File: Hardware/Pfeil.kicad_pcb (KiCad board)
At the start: 4 copper layers, 50 x 6 mm, 62 parts, among them IC1 2536030320001, IC2 nPM1300-CAAA-R, J1 Conn_01x01_Socket, J2 Conn_01x01_Socket, J3 TagConnect, U1 NRF52840-CKAA-R, U2 WSEN-PADS_2511020213301, U3 WSEN-PADS_2511020213301, X1 XTAL 32MHz 8pF, X2 XTAL 32.768kHz 9pF

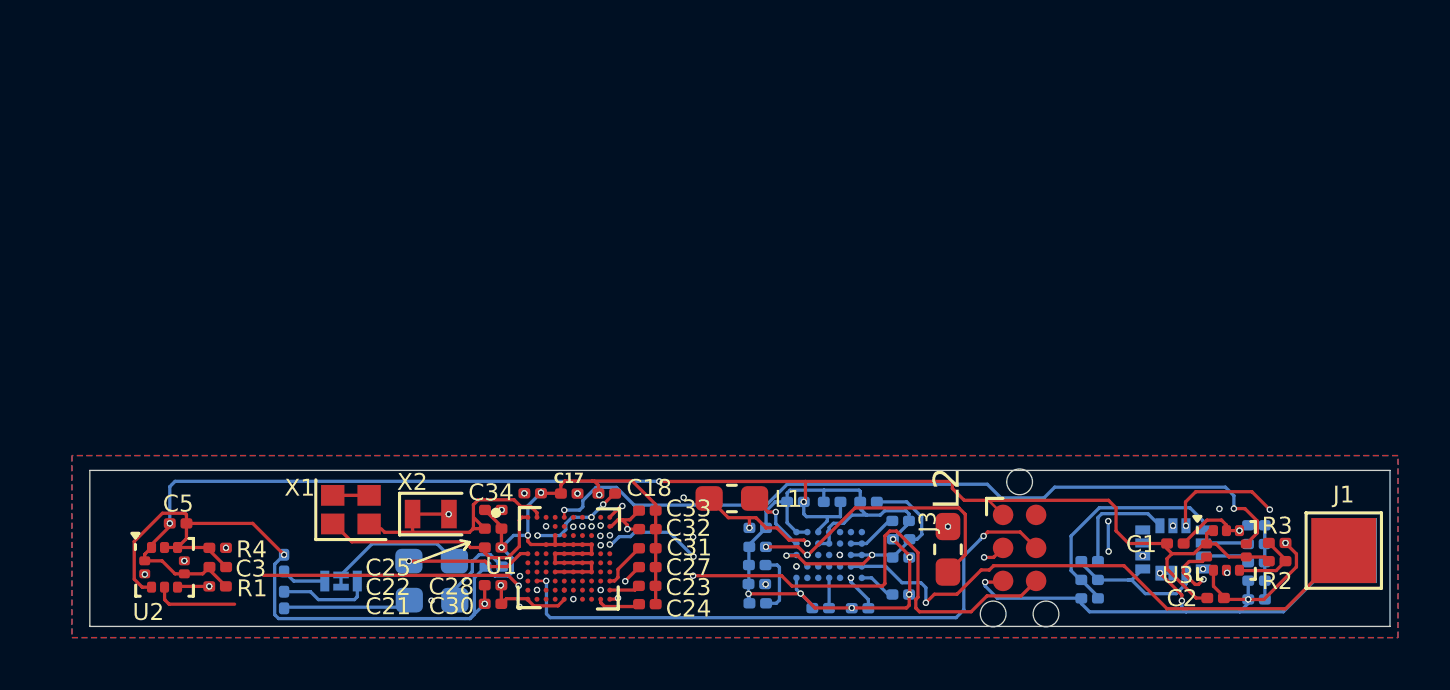
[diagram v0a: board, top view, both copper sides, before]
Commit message: Fix some shit
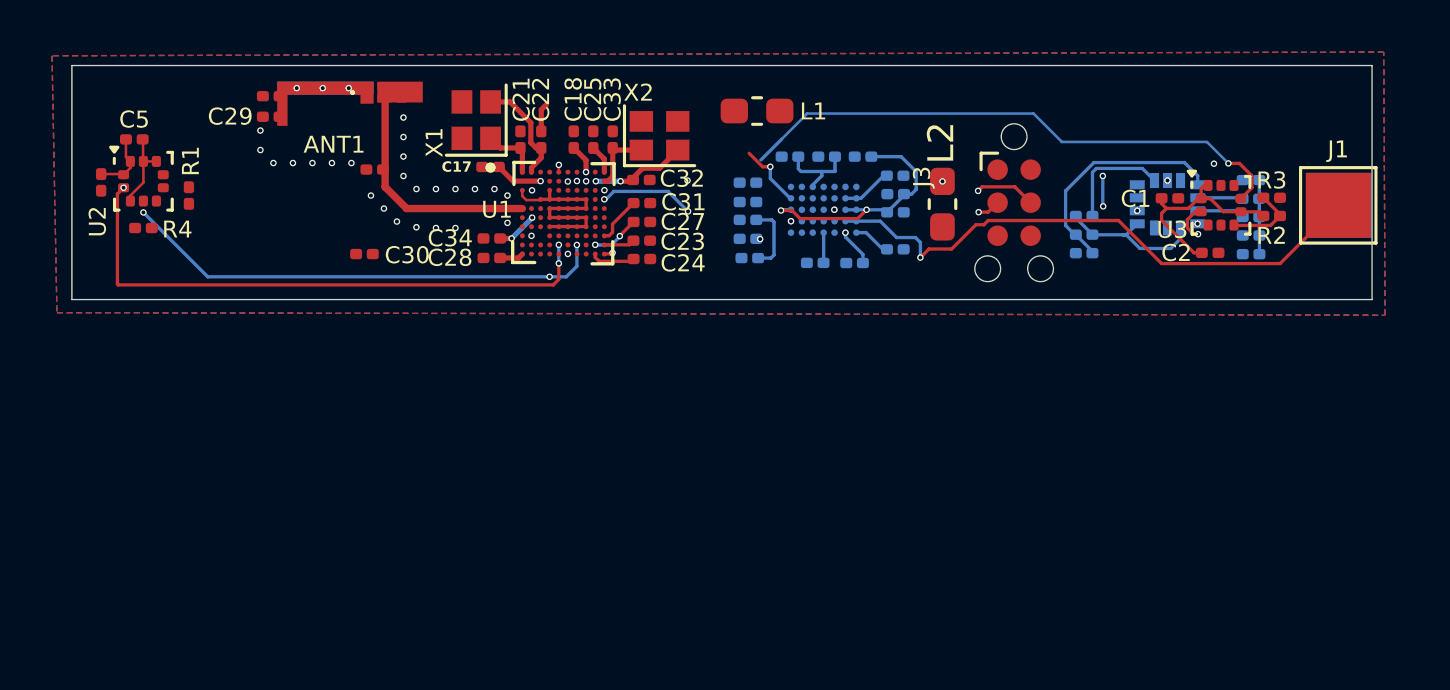
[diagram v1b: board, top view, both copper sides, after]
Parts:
- removed C26: 1.0pF NPO 5%, Capacitor_SMD:C_0201_0603Metric
- removed L5: 3.9nH 5% 0201, Inductor_SMD:L_0603_1608Metric_Pad1.05x0.95mm_HandSolder
- removed L6: 4.7nH 5% 0201, Inductor_SMD:L_0603_1608Metric_Pad1.05x0.95mm_HandSolder
- added C29: 6.2pF NPO 5%, Capacitor_SMD:C_0201_0603Metric, F.Cu at (132.7, 54.0)
- ANT1, C4, C6: moved to F.Cu
- X2: footprint Crystal:Crystal_SMD_2012-2Pin_2.0x1.2mm -> Crystal:Crystal_SMD_2016-4Pin_2.0x1.6mm
- moved ANT1 18.9 mm to (137.0, 53.0)
- moved C4 18.0 mm to (132.7, 53.2), turned to 0 degrees
- moved X2 17.0 mm to (147.6, 54.7)
- moved C6 16.9 mm to (136.6, 56.0), turned to 0 degrees
- moved X1 15.7 mm to (140.6, 54.1), turned to 90 degrees
- moved C21 15.7 mm to (142.2, 54.9), turned to 90 degrees
- moved C3 15.5 mm to (126.1, 56.5), turned to -90 degrees
- moved C22 15.1 mm to (143.1, 54.9), turned to 90 degrees
- moved R1 15.1 mm to (129.5, 57.0), turned to -90 degrees
- moved L1 14.9 mm to (151.3, 53.8)
- moved U2 14.9 mm to (127.8, 56.4)
- moved C5 14.9 mm to (127.4, 54.8)
- moved C25 14.7 mm to (145.1, 54.9), turned to -90 degrees
- moved C30 14.3 mm to (136.2, 59.2)
- moved C33 14.3 mm to (145.8, 54.9), turned to -90 degrees
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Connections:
- net Net-(ANT1-RADIATOR_ELECTRODE) renamed /RE
- ANT1 pad 2: Net-(ANT1-DUMMY_PAD_1) -> /FEEL
- ANT1 pad 3: Net-(ANT1-DUMMY_PAD_1) -> /FEEL
- ANT1 pad 4: Net-(ANT1-FEED_POINT) -> /FEEL
- C22 pad 1: Net-(U1A-P0.00/XL1) -> Net-(U1C-XC2)
- C33 pad 2: Net-(U1A-P0.00/XL1) -> Net-(U1A-P0.01/XL2)
- C6 pad 1: Net-(ANT1-FEED_POINT) -> GND
- C6 pad 2: /RF -> /FEEL
- U1 pad A2: Net-(U1A-P0.00/XL1) -> Net-(U1C-XC2)
- U1 pad B10: Net-(U1A-P0.00/XL1) -> Net-(U1A-P0.01/XL2)
- U1 pad C9: /I2C_SDA -> unconnected-(U1A-P0.26-PadC9)
- U1 pad E1: Net-(U1A-ANT) -> /FEEL
- U1 pad J5: unconnected-(U1A-P0.20-PadJ5) -> /I2C_SCL
- U1 pad J7: unconnected-(U1A-P0.14-PadJ7) -> /I2C_SDA
- X1 pad 2: Net-(U1A-P0.00/XL1) -> Net-(U1C-XC2)
- X2 pad 1: Net-(U1A-P0.00/XL1) -> Net-(U1A-P0.01/XL2)
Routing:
- net GND: track 114.4 -> 16.9 mm, vias 21 -> 26
- net /I2C_SDA: track 82.6 -> 18.7 mm, vias 6 -> 3
- net +3V3: track 60.0 -> 13.7 mm, vias 3 -> 0
- net /I2C_SCL: track 79.6 -> 53.7 mm
- net /SWDIO: track 25.3 -> 0.00 mm, vias 2 -> 0
- net /SWCLK: track 23.5 -> 2.48 mm
- net Net-(U1A-P0.00/XL1): track 23.0 -> 4.51 mm, vias 3 -> 2
- net /PADS_INT01: track 16.4 -> 0.02 mm, vias 2 -> 1
- net /3.0V: track 11.1 -> 0.00 mm, vias 2 -> 0
- net Net-(ANT1-DUMMY_PAD_1): track 9.63 -> 0.00 mm
- net /FEEL: track 0.00 -> 9.02 mm
- net /PADS_INT02: track 30.3 -> 22.0 mm
- net Net-(U1C-XC1): track 9.41 -> 2.26 mm
- net VDD: track 22.7 -> 17.5 mm, vias 4 -> 2
- net /RF: track 4.95 -> 0.00 mm
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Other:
- board size 50 x 6 mm -> 50 x 9 mm
